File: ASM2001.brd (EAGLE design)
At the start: 22.5 x 22.5 mm, 19 parts, among them J1 3013, J2 DF12-32-DP, Q1 NTZD3152P, Q2 2N7002P, SW1 APTCLG, U1 ATMEGA328P, Y1 8MHz

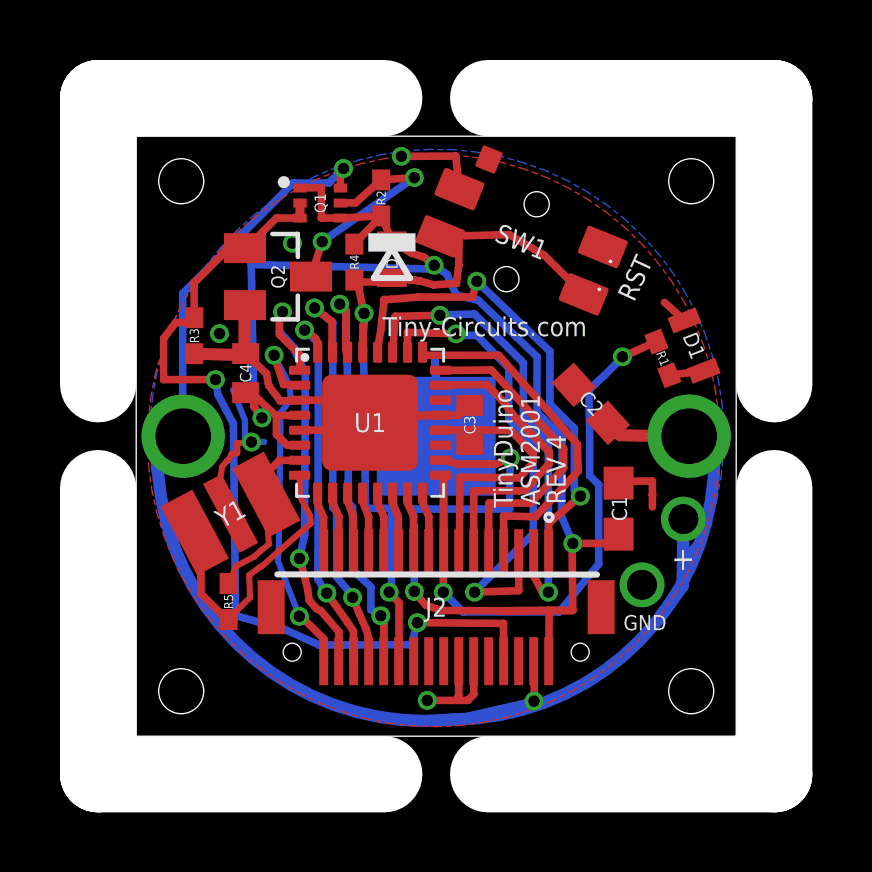
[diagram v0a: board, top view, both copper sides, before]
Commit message: Updated to Rev6
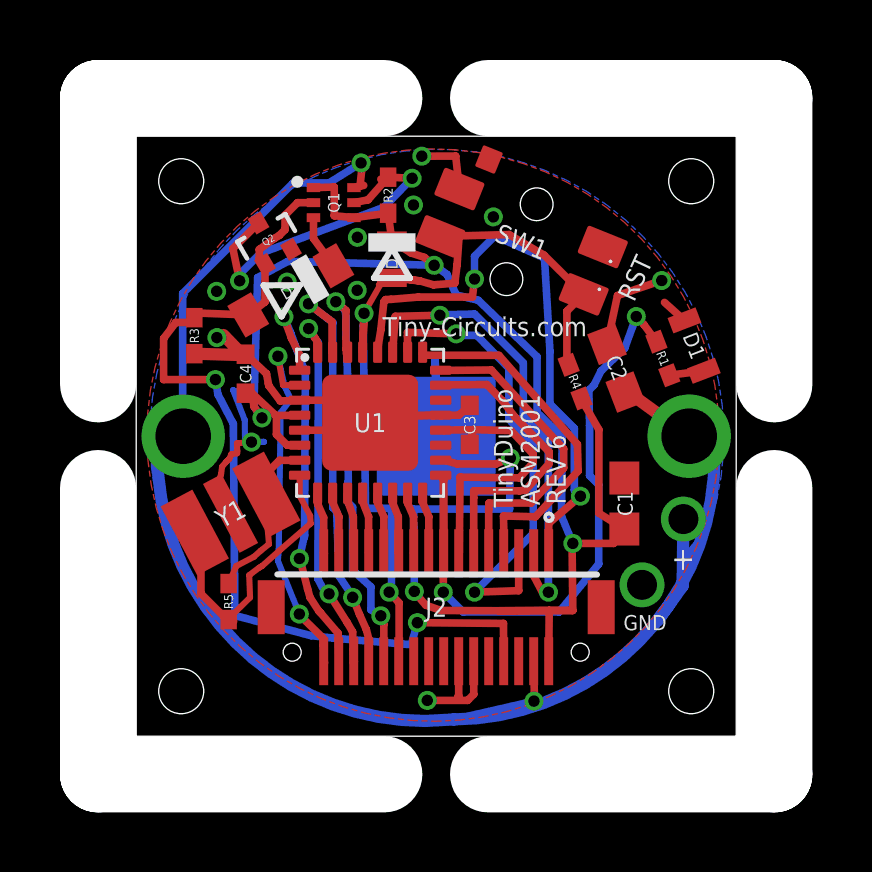
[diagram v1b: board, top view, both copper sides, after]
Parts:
- added D3: MBR120, tinycircuits:SOD-123FL
- Q2: value 2N7002P -> 2N7002PT; device tinycircuits:SOT23 -> tinycircuits:SOT-416
- moved R4 8.37 mm to (24.6, 21.8), turned to 291 degrees
- moved C2 1.46 mm to (26.0, 22.3), turned to 111 degrees
- moved Q2 1.27 mm to (14.4, 26.5), turned to 30 degrees
- moved Q1 0.45 mm to (16.6, 27.8)
- moved C1 0.26 mm to (26.3, 17.8)
- moved R2 0.25 mm to (18.4, 28.0)
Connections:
- new net N$2: D3.C, Q1.3
- net +5V: now also D3.A; no longer Q1.3
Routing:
- net N$8: track 7.75 -> 11.8 mm
- net AD5/SCL: track 16.3 -> 19.6 mm
- net VCC: track 59.2 -> 62.2 mm
- net N$2: track 0.00 -> 1.82 mm
- net RESET: track 27.6 -> 29.3 mm
- net SCK: track 22.3 -> 23.5 mm
- net +5V: track 29.6 -> 30.4 mm
- net IO3: track 15.0 -> 14.2 mm
- net VBATT: track 57.4 -> 58.1 mm
- net GND: track 36.9 -> 36.6 mm, vias 6 -> 12
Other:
- board text added: "6"
- board text added: "REV 6"
- board text removed: "4"
- board text removed: "REV 4"

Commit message: Updated to Rev 8
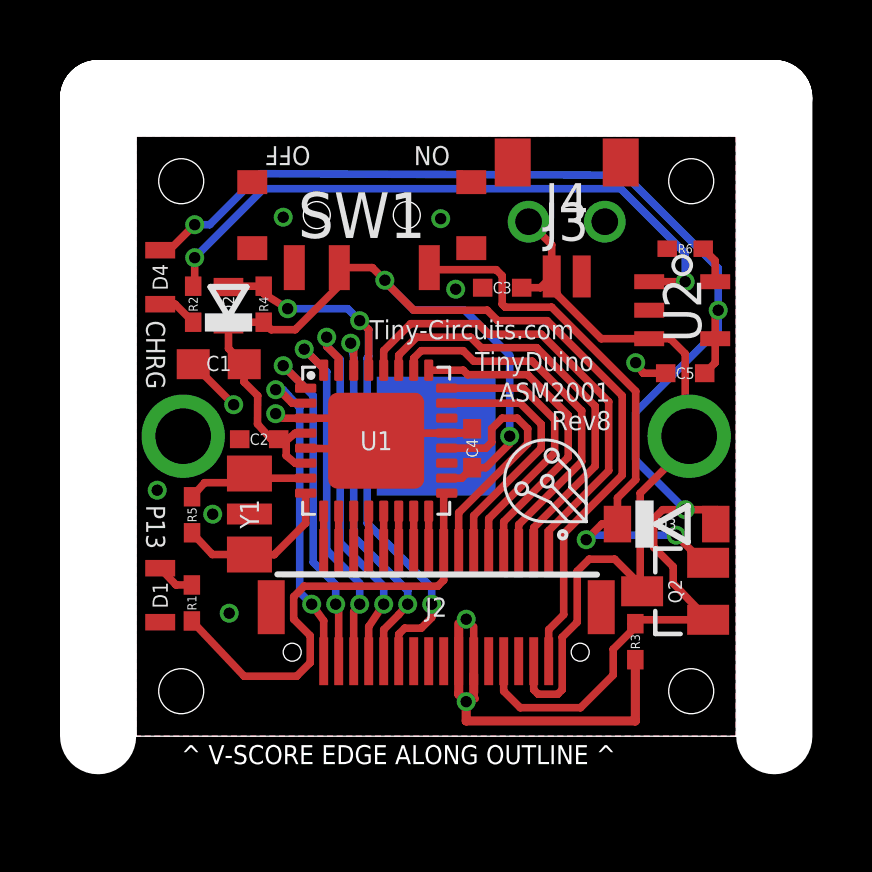
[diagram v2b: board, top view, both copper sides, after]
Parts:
- removed Q1: NTZD3152P, tinycircuits:SOT-563-6
- added C5: 4.7uF, tinycircuits:C0402
- added D4: AMBER, tinycircuits:LNJ_LED
- added J3: 961102, tinycircuits:2X.1"
- added J4: SM02B-SRSS-TB(LF)(SN), tinycircuits:JST_SH_2X1
- added R6: 10K, tinycircuits:0402
- added U2: MCP73831, tinycircuits:SOT-23
- C2: value 10uF -> .1uF; device tinycircuits:C0603 -> tinycircuits:C0402
- C3: value .1uF -> 4.7uF
- Q2: value 2N7002PT -> DMP2035U; device tinycircuits:SOT-416 -> tinycircuits:SOT23
- R2: value 100k -> 1k
- SW1: value APTCLG -> PCM12SMTR; device tinycircuits:APTCLGTVTR -> tinycircuits:PCM12SMTR
- Y1: value 8MHz -> 8.00MHZ; device tinycircuits:RESONATOR -> tinycircuits:RESONATOR_SMALL
- moved D1 19.6 mm to (10.8, 14.7), turned to 0 degrees
- moved Q2 17.9 mm to (28.0, 14.8), turned to 90 degrees
- moved R3 17.9 mm to (26.6, 13.2)
- moved R1 17.7 mm to (11.9, 14.4), turned to 270 degrees
- moved D3 14.8 mm to (27.7, 17.1), turned to 0 degrees
- moved C1 14.3 mm to (12.8, 22.4), turned to 180 degrees
- moved C2 12.1 mm to (14.1, 19.9), turned to 180 degrees
- moved R4 10.7 mm to (14.2, 24.4), turned to 270 degrees
- moved C4 7.95 mm to (21.2, 19.6)
- moved R2 7.44 mm to (11.9, 24.4), turned to 90 degrees
- moved D2 5.66 mm to (13.1, 24.4), turned to 90 degrees
- moved SW1 5.40 mm to (17.5, 27.4), turned to 180 degrees
- moved C3 4.70 mm to (22.2, 24.9), turned to 180 degrees
- moved R5 3.14 mm to (11.9, 17.4)
- moved U1 0.63 mm to (18.0, 19.9)
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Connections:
- removed net N$8: Q1.5, Q2.3, R2.1
- new net 1: J1.1
- new net N$5: D4.C, R2.1
- new net N$6: R6.1, U2.5
- new net N$7: R2.2, U2.1
- net +5V: now also C5.1, D4.A, Q2.B, U2.4; no longer Q1.2, Q2.1
- net AREF: no longer C3.1
- net GND: now also C5.2, J3.2, J4.1, R6.2, SW1.W1, SW1.W2, SW1.W3, SW1.W4, U2.2; no longer Q2.2, SW1.2, SW1.4, SW1.5
- net N$2: now also Q2.E, SW1.1; no longer Q1.3
- net RESET: no longer SW1.1, SW1.3
- net VBATT: now also C3.1, J3.1, J4.2, Q2.C, U2.3; no longer C2.1, J1.1, Q1.6
- net VCC: now also C2.1, SW1.2; no longer Q1.1, Q1.4, R2.2
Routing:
- net VBATT: track 58.1 -> 26.7 mm, vias 3 -> 0
- net N$7: track 0.00 -> 21.3 mm, vias 0 -> 2
- net +5V: track 30.4 -> 49.9 mm, vias 2 -> 3
- net VCC: track 62.2 -> 44.4 mm, vias 5 -> 2
- net N$2: track 1.82 -> 19.6 mm, vias 0 -> 2
- net N$8: track 11.8 -> 0.00 mm, vias 2 -> 0
- net RESET: track 29.3 -> 20.1 mm, vias 2 -> 3
- net GND: track 36.6 -> 28.3 mm, vias 12 -> 11
- net SCK: track 23.5 -> 15.5 mm, vias 2 -> 0
- net N$1: track 9.95 -> 5.54 mm
- net AD5/SCL: track 19.6 -> 15.5 mm, vias 2 -> 0
- net AD3: track 15.9 -> 12.6 mm, vias 2 -> 0
- net IO3: track 14.2 -> 11.7 mm
- net IO4: track 13.3 -> 11.0 mm
- net IO0: track 14.7 -> 12.6 mm
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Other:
- board size 22.5 x 22.5 mm -> 22.5 x 21.3 mm
- board text added: "-"
- board text added: "8"
- board text added: "CHRG"
- board text added: "OFF"
- board text added: "ON"
- board text added: "P13"
- board text added: "Rev8"
- board text added: "^ V-SCORE EDGE ALONG OUTLINE ^"
- board text removed: "6"
- board text removed: "GND"
- board text removed: "REV 6"
- board text removed: "RST"
